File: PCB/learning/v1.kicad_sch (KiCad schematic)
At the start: 8 parts, among them U1 STM32F100C4Tx

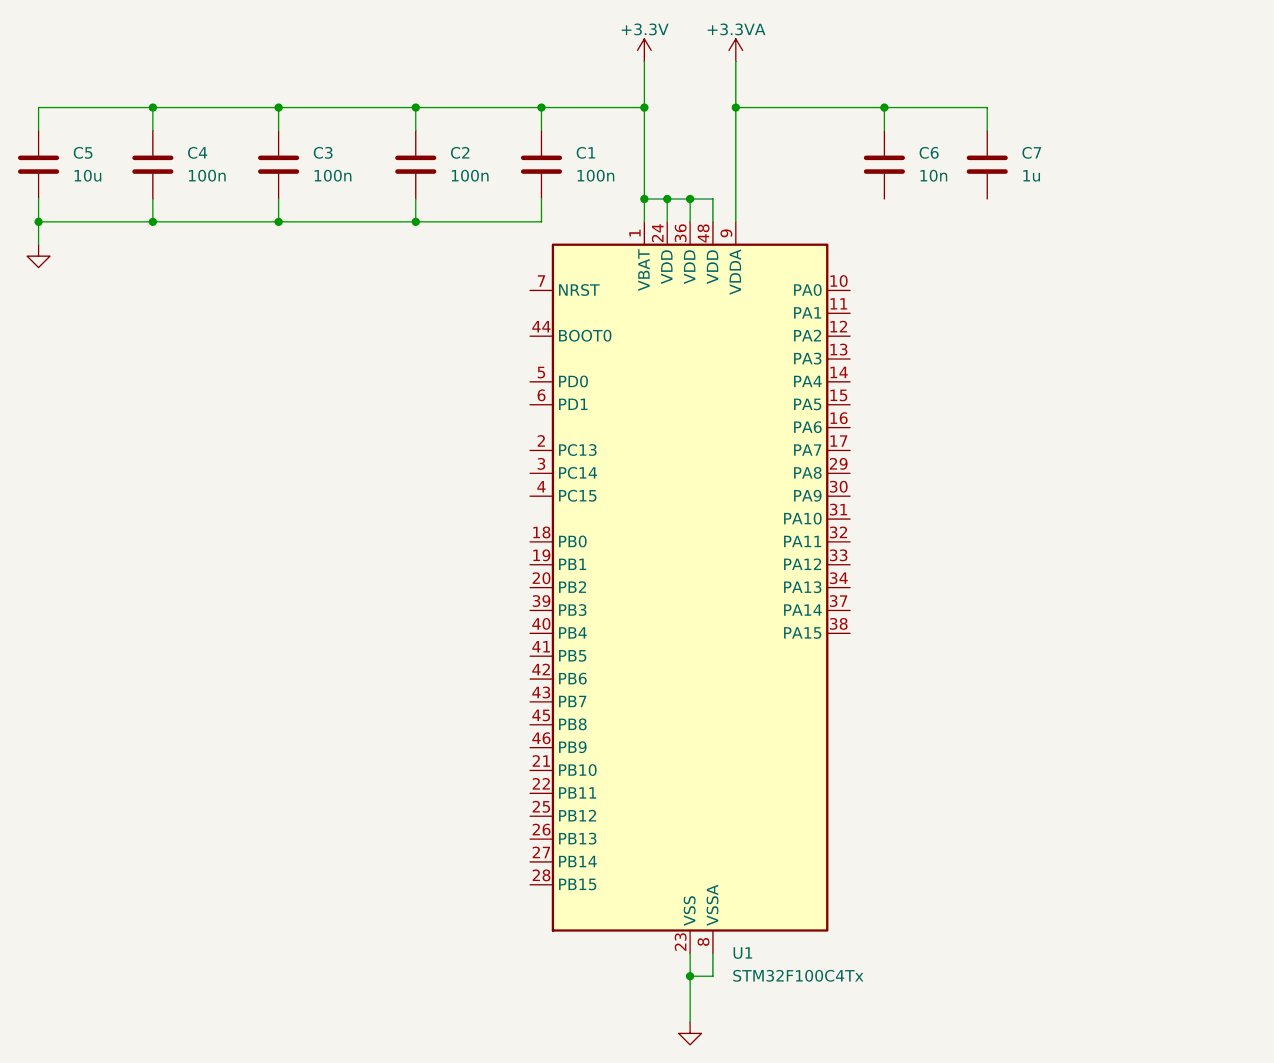
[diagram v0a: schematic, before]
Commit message: PCB v0.1: barebones setup
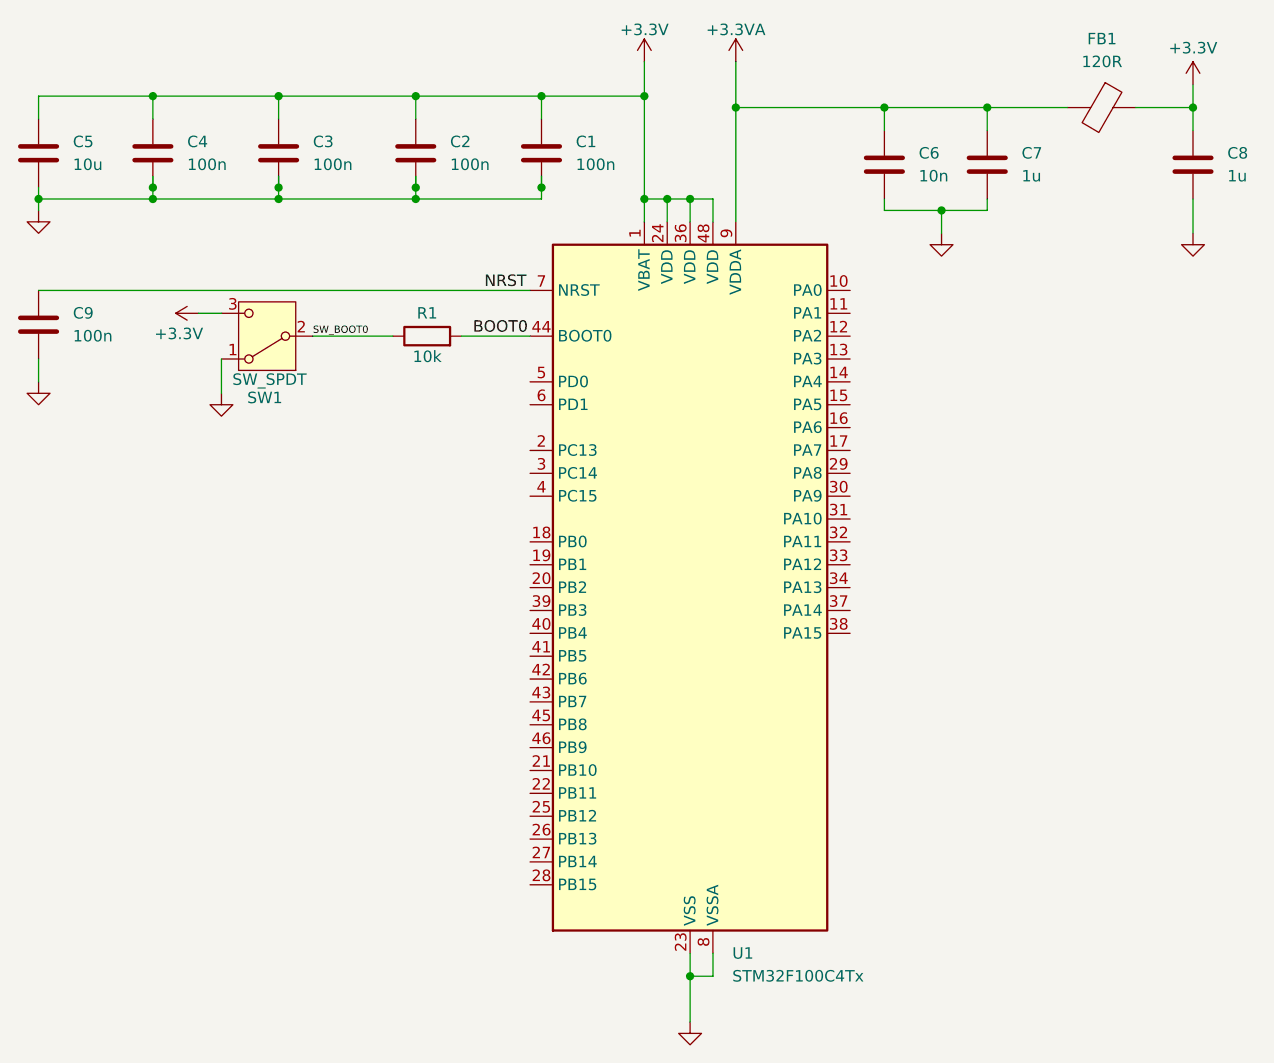
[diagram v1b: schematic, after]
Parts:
- added C8: 1u, symbol Device:C
- added C9: 100n, symbol Device:C
- added FB1: 120R, symbol Device:FerriteBead
- added R1: 10k, symbol Device:R
- added SW1: SW_SPDT, symbol Switch:SW_SPDT
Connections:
- net +3.3V: now also C8.1, FB1.1, SW1.3 (C)
- net +3.3VA: now also FB1.2
- net GND: now also C6.2, C7.2, C8.2, C9.2, SW1.1 (A)
- net BOOT0: now reaches U1.44 (BOOT0)
- net BOOT0: now also R1.2
- net NRST: now reaches U1.7 (NRST)
- net NRST: now also C9.1
- new net SW_BOOT0: R1.1, SW1.2 (B)
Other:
- moved on the sheet: C1, C2, C3, C4, C5
